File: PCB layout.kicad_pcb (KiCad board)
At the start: 2 copper layers, 90 x 64 mm, 15 parts, among them J2 Conn_01x02_Male, Q1 2P222

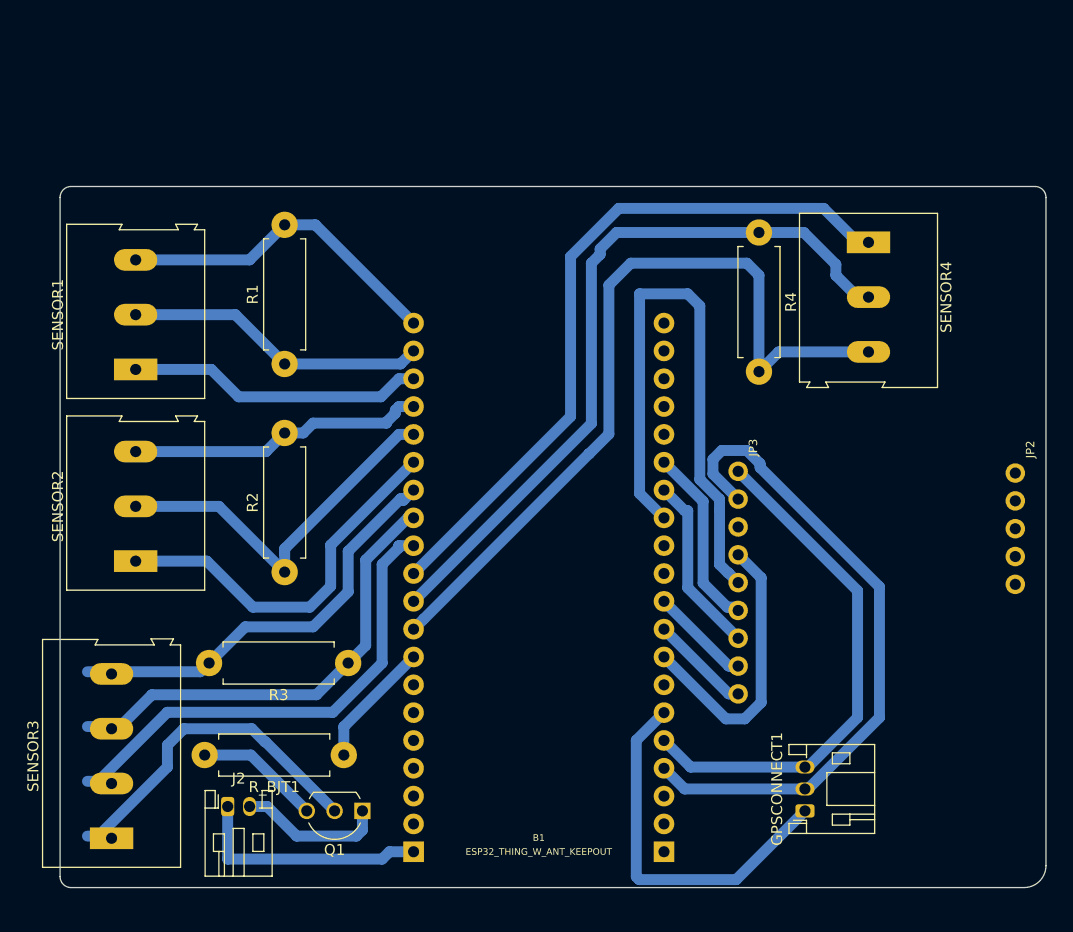
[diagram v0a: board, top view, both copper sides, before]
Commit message: Version 1.1
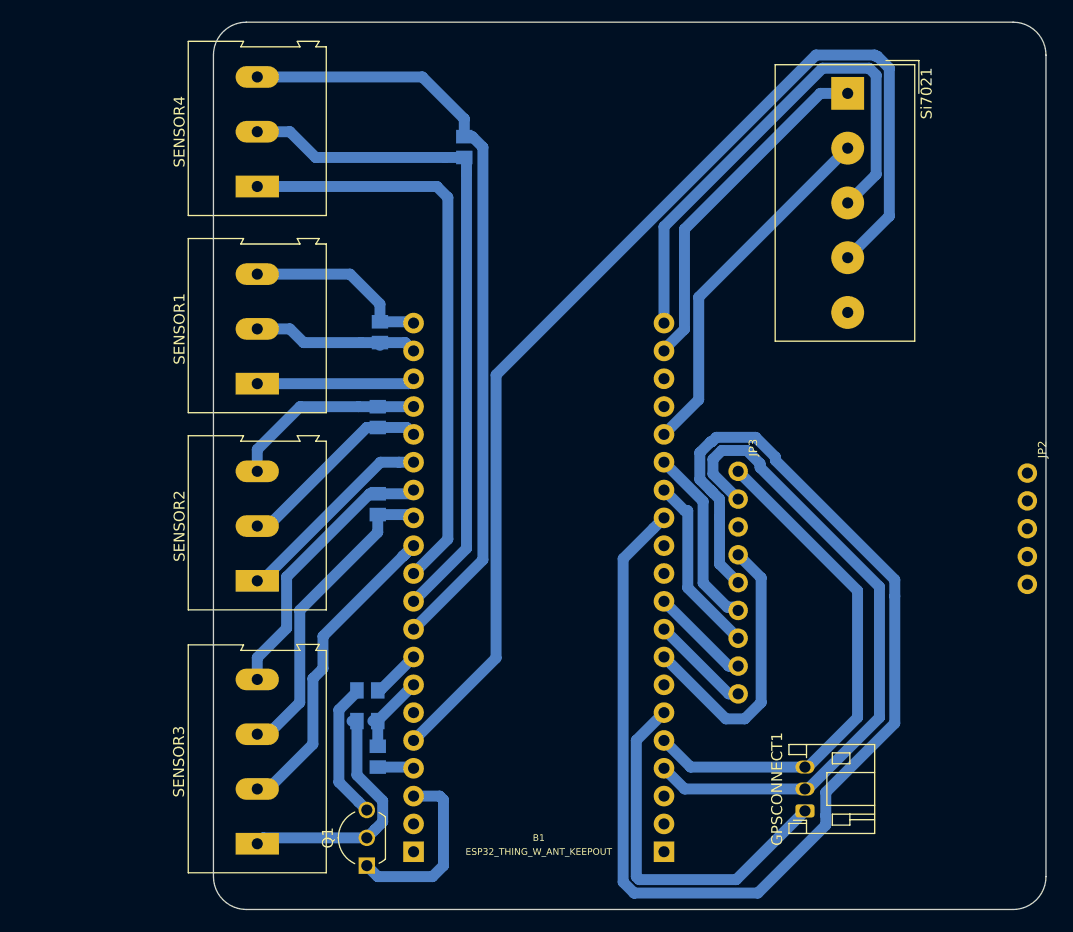
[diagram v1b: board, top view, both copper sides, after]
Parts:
- removed J2: Conn_01x02_Male, Connector_JST:JST_PH_S2B-PH-K_1x02_P2.00mm_Horizontal
- added RBAT1: 100K, Adafruit RFM+LoRa Breakout:0805-NO, B.Cu at (222.1, 79.8)
- added RBAT2: 27K, Adafruit RFM+LoRa Breakout:0805-NO, B.Cu at (223.0, 83.0)
- added Si7021: HEADER-1X570MIL, TerminalBlock_Altech:Altech_AK300_1x05_P5.00mm_45-Degree, F.Cu at (265.9, 22.5)
- R1, R2, R3, R4, R_BJT1: footprint Resistor_THT:R_Axial_DIN0411_L9.9mm_D3.6mm_P12.70mm_Horizontal -> Adafruit RFM+LoRa Breakout:0805-NO; moved to B.Cu
- moved SENSOR4 56.0 mm to (212.0, 31.0), turned to 90 degrees
- moved R4 28.0 mm to (230.9, 27.4), turned to 90 degrees
- moved R2 16.5 mm to (223.0, 52.0)
- moved R3 14.7 mm to (223.0, 60.0), turned to 90 degrees
- moved SENSOR3 13.3 mm to (212.0, 91.0)
- moved SENSOR2 11.2 mm to (212.0, 67.0)
- moved SENSOR1 11.2 mm to (212.0, 49.0)
- moved R1 9.17 mm to (223.2, 44.3)
- moved R_BJT1 6.28 mm to (222.1, 77.0)
- moved Q1 5.02 mm to (222.0, 93.0), turned to 90 degrees
- moved JP2 1.10 mm to (282.3, 62.2)
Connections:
- B1 pad 21: Net-(B1-Pad21) -> /GND
- B1 pad 22: Net-(B1-Pad22) -> /SDA
- B1 pad 25: Net-(B1-Pad25) -> /SCL
- B1 pad 36: VIN -> /VCC
- B1 pad 37: GND -> /GND
- B1 pad 5: Net-(B1-Pad5) -> /+3V3
- GPSCONNECT1 pad 2: GND -> /GND
- GPSCONNECT1 pad 3: VIN -> /VCC
- Q1 pad 1: Net-(J2-Pad2) -> Net-(B1-Pad3)
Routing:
- net /+3V3: track 0.00 -> 103.9 mm
- net /SCK_5V: track 54.1 -> 118.6 mm
- net /GND: track 0.00 -> 49.8 mm
- net /SCL: track 0.00 -> 33.1 mm
- net /SDA: track 0.00 -> 31.9 mm
- net Net-(B1-Pad1): track 22.0 -> 0.00 mm
- net Net-(B1-Pad16): track 35.3 -> 18.3 mm
- net Net-(B1-Pad15): track 35.8 -> 18.8 mm
- net Net-(B1-Pad3): track 0.00 -> 16.7 mm
- net Net-(B1-Pad12): track 44.1 -> 30.1 mm
- net Net-(B1-Pad18): track 28.1 -> 14.5 mm
- net Net-(B1-Pad14): track 39.0 -> 25.5 mm
- net Net-(J2-Pad2): track 13.4 -> 0.00 mm
- net Net-(B1-Pad20): track 30.4 -> 17.1 mm
- net Net-(B1-Pad13): track 42.2 -> 29.1 mm
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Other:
- board size 90 x 64 mm -> 76 x 81 mm
